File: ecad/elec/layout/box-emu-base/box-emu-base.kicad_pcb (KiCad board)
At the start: 2 copper layers, 72.5 x 63.9 mm, 69 parts

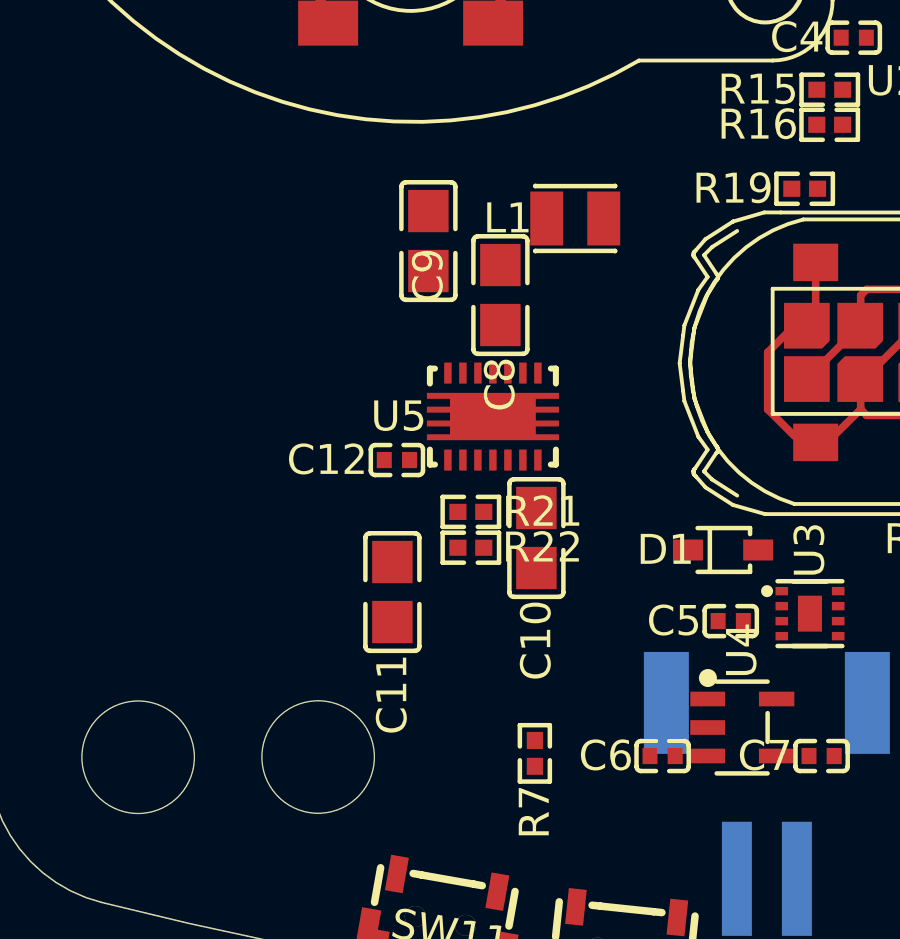
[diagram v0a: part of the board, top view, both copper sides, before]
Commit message: further layout changes
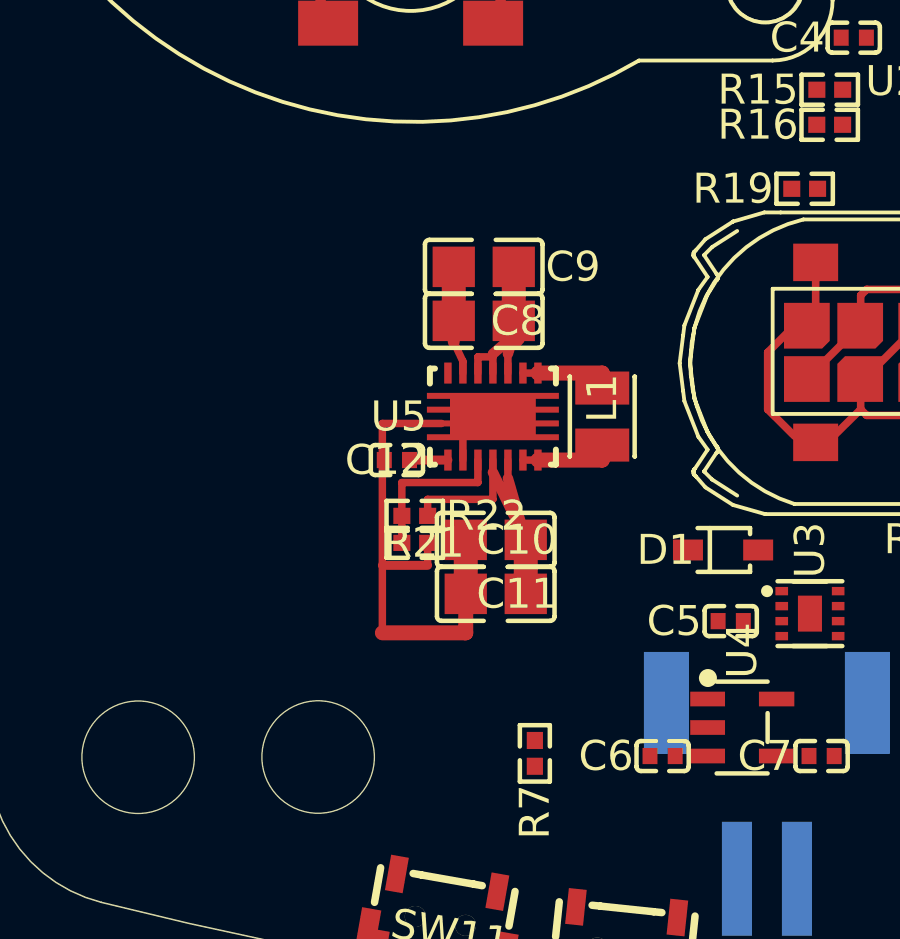
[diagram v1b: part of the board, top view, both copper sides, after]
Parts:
- moved L1 6.66 mm to (120.0, 118.6), turned to 270 degrees
- moved C11 3.45 mm to (116.4, 124.5), turned to 180 degrees
- moved R22 2.15 mm to (113.7, 121.9)
- moved R21 2.14 mm to (113.7, 122.8), turned to 0 degrees
- moved C9 2.04 mm to (116.0, 113.6), turned to 180 degrees
- moved C10 1.36 mm to (116.4, 122.7), turned to 180 degrees
- moved C8 1.02 mm to (116.0, 115.4), turned to 180 degrees
- turned C12 to 180 degrees
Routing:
- net gnd: track 0.00 -> 21.5 mm
- net vcc_5v: track 0.00 -> 11.1 mm
- net vbat: track 0.00 -> 7.45 mm
- net FB: track 0.00 -> 5.30 mm
- net 2: track 0.00 -> 3.14 mm
- net 1: track 0.00 -> 3.14 mm
